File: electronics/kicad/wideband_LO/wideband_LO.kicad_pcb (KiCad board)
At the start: 2 copper layers, 27 parts, among them U1 BFP620

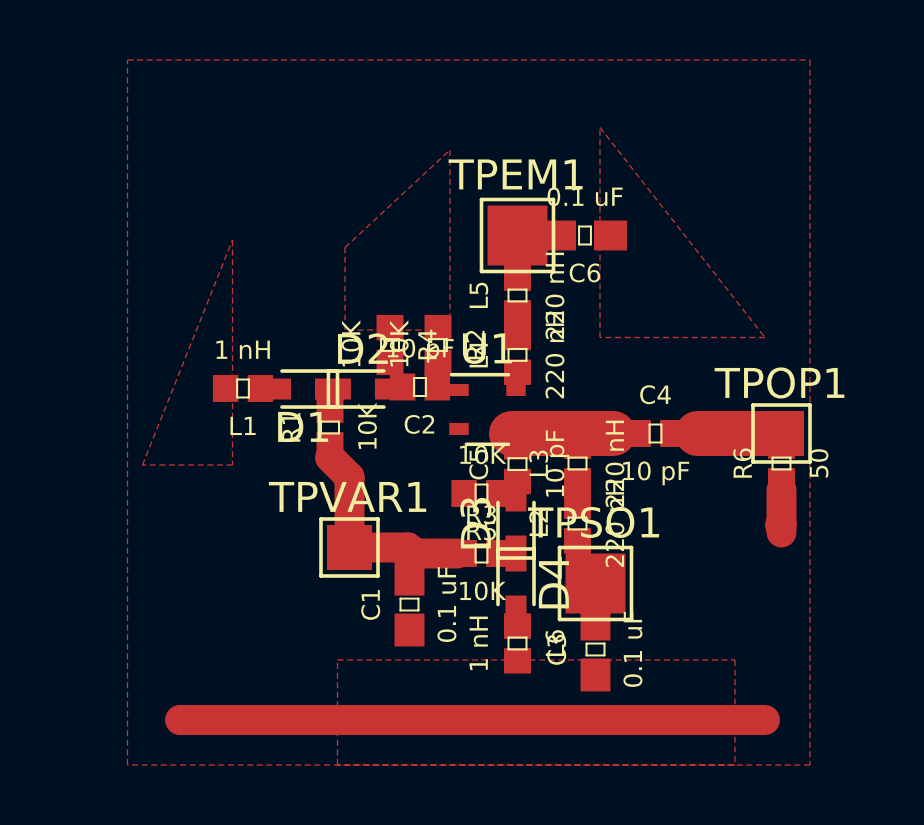
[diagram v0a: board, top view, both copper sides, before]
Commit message: Various sims
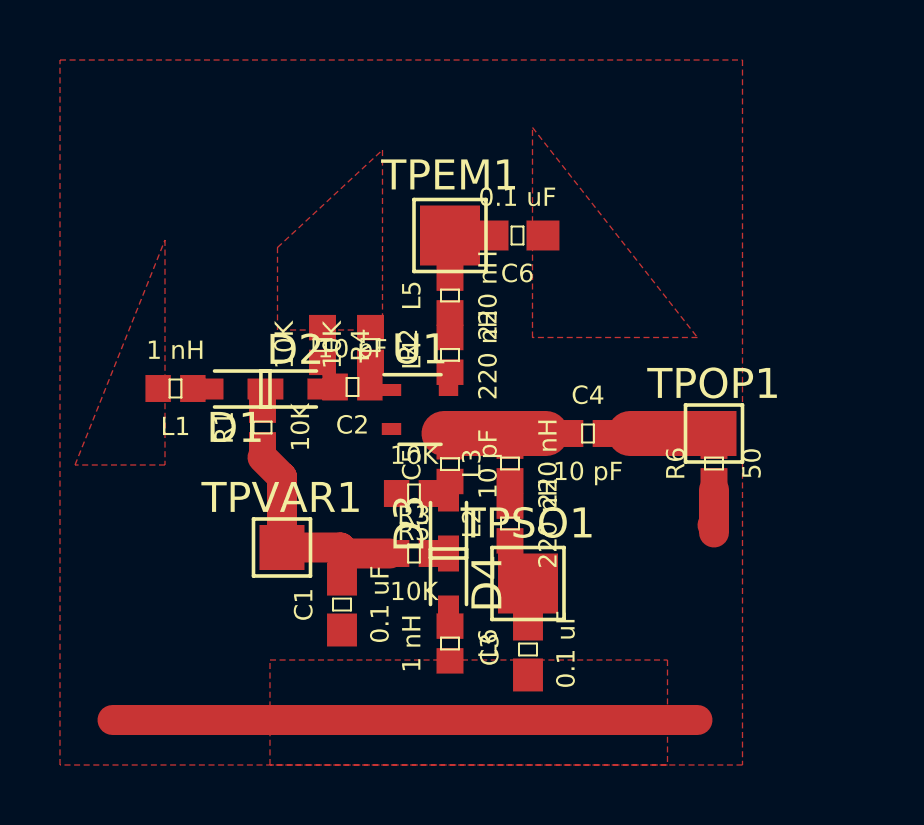
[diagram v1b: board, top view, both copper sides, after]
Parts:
- moved C1 2.25 mm to (93.2, 103.9)
- moved C2 2.25 mm to (93.5, 96.7)
- moved C3 2.25 mm to (99.3, 105.4)
- moved C4 2.25 mm to (101.3, 98.2)
- moved C5 2.25 mm to (96.8, 99.2)
- moved C6 2.25 mm to (99.0, 91.6)
- moved D1 2.25 mm to (89.6, 96.7)
- moved D2 2.25 mm to (91.6, 96.7)
- moved D3 2.25 mm to (96.7, 101.2)
- moved D4 2.25 mm to (96.7, 103.2)
- moved L1 2.25 mm to (87.6, 96.7)
- moved L2 2.25 mm to (98.8, 101.2)
- moved L3 2.25 mm to (98.8, 99.2)
- moved L4 2.25 mm to (96.8, 95.6)
- moved L5 2.25 mm to (96.8, 93.6)
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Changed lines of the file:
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@@
     (visible_elements FFFFFF7F)
     (pcbplotparams
-      (layerselection 0x010fc_ffffffff)
+      (layerselection 0x00000_7fffffff)
       (usegerberextensions false)
       (usegerberattributes false)
@@
       (creategerberjobfile false)
       (excludeedgelayer true)
-      (linewidth 0.010000)
+      (linewidth 0.020000)
       (plotframeref false)
       (viasonmask false)
       (mode 1)
-      (useauxorigin false)
+      (useauxorigin true)
       (hpglpennumber 1)
       (hpglpenspeed 20)
@@
       (outputformat 1)
       (mirror false)
-      (drillshape 1)
+      (drillshape 0)
       (scaleselection 1)
-      (outputdirectory ""))
+      (outputdirectory "CAM/"))
   )
   (net 0 "")
@@
   )
   (module Capacitors:0402 (layer F.Cu)
-    (at 107.8 99.2 90)
+    (at 105.55 99.2 90)
     (descr "GENERIC 1005 (0402) PACKAGE")
     (tags "GENERIC 1005 (0402) PACKAGE")
@@
   )
   (module Capacitors:0402 (layer F.Cu)
-    (at 97.8 100.2 180)
+    (at 95.55 100.2 180)
     (descr "GENERIC 1005 (0402) PACKAGE")
     (tags "GENERIC 1005 (0402) PACKAGE")
@@
   )
   (module Capacitors:0402 (layer F.Cu)
-    (at 94.75 95.25 270)
+    (at 92.5 95.25 270)
     (descr "GENERIC 1005 (0402) PACKAGE")
     (tags "GENERIC 1005 (0402) PACKAGE")
@@
   )
   (module Capacitors:0402 (layer F.Cu)
-    (at 97.8 102.2)
+    (at 95.55 102.2)
     (descr "GENERIC 1005 (0402) PACKAGE")
     (tags "GENERIC 1005 (0402) PACKAGE")
@@
   )
   (module Capacitors:0402 (layer F.Cu)
-    (at 96.35 95.25 270)
+    (at 94.1 95.25 270)
     (descr "GENERIC 1005 (0402) PACKAGE")
     (tags "GENERIC 1005 (0402) PACKAGE")
@@
   )
   (module Capacitors:0402 (layer F.Cu)
-    (at 92.75 98 90)
+    (at 90.5 98 90)
     (descr "GENERIC 1005 (0402) PACKAGE")
     (tags "GENERIC 1005 (0402) PACKAGE")
@@
   )
   (module Capacitors:0402 (layer F.Cu)
-    (at 99 105.2 270)
+    (at 96.75 105.2 270)
     (descr "GENERIC 1005 (0402) PACKAGE")
     (tags "GENERIC 1005 (0402) PACKAGE")
@@
   )
   (module Capacitors:0402 (layer F.Cu)
-    (at 99 93.6 90)
+    (at 96.75 93.6 90)
     (descr "GENERIC 1005 (0402) PACKAGE")
     (tags "GENERIC 1005 (0402) PACKAGE")
@@
   )
   (module Capacitors:0402 (layer F.Cu)
-    (at 99 95.57912 90)
+    (at 96.75 95.57912 90)
     (descr "GENERIC 1005 (0402) PACKAGE")
     (tags "GENERIC 1005 (0402) PACKAGE")
@@
   )
   (module Capacitors:0402 (layer F.Cu)
-    (at 101 99.2 90)
+    (at 98.75 99.2 90)
     (descr "GENERIC 1005 (0402) PACKAGE")
     (tags "GENERIC 1005 (0402) PACKAGE")
@@
   )
   (module Capacitors:0402 (layer F.Cu)
-    (at 101 101.2 90)
+    (at 98.75 101.2 90)
     (descr "GENERIC 1005 (0402) PACKAGE")
     (tags "GENERIC 1005 (0402) PACKAGE")
@@
   )
   (module Capacitors:0402 (layer F.Cu)
-    (at 89.85 96.7 180)
+    (at 87.6 96.7 180)
     (descr "GENERIC 1005 (0402) PACKAGE")
     (tags "GENERIC 1005 (0402) PACKAGE")
@@
   )
   (module Capacitors:0603 (layer F.Cu)
-    (at 101.25 91.6 180)
+    (at 99 91.6 180)
     (descr "GENERIC 1608 (0603) PACKAGE")
     (tags "GENERIC 1608 (0603) PACKAGE")
@@
   )
   (module Capacitors:0402 (layer F.Cu)
-    (at 99 99.22088 90)
+    (at 96.75 99.22088 90)
     (descr "GENERIC 1005 (0402) PACKAGE")
     (tags "GENERIC 1005 (0402) PACKAGE")
@@
   )
   (module Capacitors:0402 (layer F.Cu)
-    (at 103.6 98.2)
+    (at 101.35 98.2)
     (descr "GENERIC 1005 (0402) PACKAGE")
     (tags "GENERIC 1005 (0402) PACKAGE")
@@
   )
   (module Capacitors:0603 (layer F.Cu)
-    (at 101.6 105.4 90)
+    (at 99.35 105.4 90)
     (descr "GENERIC 1608 (0603) PACKAGE")
     (tags "GENERIC 1608 (0603) PACKAGE")
@@
   )
   (module Capacitors:0402 (layer F.Cu)
-    (at 95.75 96.65 180)
+    (at 93.5 96.65 180)
     (descr "GENERIC 1005 (0402) PACKAGE")
     (tags "GENERIC 1005 (0402) PACKAGE")
@@
   )
   (module Capacitors:0603 (layer F.Cu)
-    (at 95.4 103.90164 90)
+    (at 93.15 103.90164 90)
     (descr "GENERIC 1608 (0603) PACKAGE")
     (tags "GENERIC 1608 (0603) PACKAGE")
@@
   )
   (module TestPoint:TestPoint_Pad_1.5x1.5mm (layer F.Cu)
-    (at 93.4 102)
+    (at 91.15 102)
     (descr "SMD rectangular pad as test Point, square 1.5mm side length")
     (tags "test point SMD pad rectangle square")
@@
   )
   (module Diode_SMD:D_SOD-523 (layer F.Cu)
-    (at 93.847057 96.717156)
+    (at 91.597057 96.717156)
     (descr "http://www.diodes.com/datasheets/ap02001.pdf p.144")
     (tags "Diode SOD523")
@@
   )
   (module Diode_SMD:D_SOD-523 (layer F.Cu)
-    (at 98.95 101.2 90)
+    (at 96.7 101.2 90)
     (descr "http://www.diodes.com/datasheets/ap02001.pdf p.144")
     (tags "Diode SOD523")
@@
   )
   (module Diode_SMD:D_SOD-523 (layer F.Cu)
-    (at 91.85 96.717157 180)
+    (at 89.6 96.717157 180)
     (descr "http://www.diodes.com/datasheets/ap02001.pdf p.144")
     (tags "Diode SOD523")
@@
   )
   (module Diode_SMD:D_SOD-523 (layer F.Cu)
-    (at 98.95 103.199999 270)
+    (at 96.7 103.199999 270)
     (descr "http://www.diodes.com/datasheets/ap02001.pdf p.144")
     (tags "Diode SOD523")
@@
   )
   (module Package_TO_SOT_SMD:SOT-343_SC-70-4 (layer F.Cu)
-    (at 98 97.4)
+    (at 95.75 97.4)
     (descr "SOT-343, SC-70-4")
     (tags "SOT-343 SC-70-4")
@@
   )
   (module TestPoint:TestPoint_Pad_2.0x2.0mm (layer F.Cu)
-    (at 99 91.6)
+    (at 96.75 91.6)
     (descr "SMD rectangular pad as test Point, square 2.0mm side length")
     (tags "test point SMD pad rectangle square")
@@
   )
   (module TestPoint:TestPoint_Pad_2.0x2.0mm (layer F.Cu)
-    (at 101.6 103.2)
+    (at 99.35 103.2)
     (descr "SMD rectangular pad as test Point, square 2.0mm side length")
     (tags "test point SMD pad rectangle square")
@@
   )
   (module TestPoint:TestPoint_Pad_1.5x1.5mm (layer F.Cu)
-    (at 107.8 98.2)
+    (at 105.55 98.2)
     (descr "SMD rectangular pad as test Point, square 1.5mm side length")
     (tags "test point SMD pad rectangle square")
@@
       (net 15 noutput))
   )
-  (segment (start 87.75 107.75) (end 107.25 107.75) (width 1) (layer F.Cu) (net 1))
-  (segment (start 95.35164 102) (end 95.4 102.04836) (width 1) (layer F.Cu) (net 14))
-  (segment (start 93.4 102) (end 95.35164 102) (width 1) (layer F.Cu) (net 14))
-  (segment (start 95.55164 102.2) (end 95.4 102.04836) (width 1) (layer F.Cu) (net 14))
-  (segment (start 97 102.2) (end 95.33076 102.2) (width 1) (layer F.Cu) (net 14))
-  (segment (start 93.4 102) (end 93.4 99.65) (width 1) (layer F.Cu) (net 14))
-  (segment (start 93.4 99.65) (end 92.75 99) (width 1) (layer F.Cu) (net 14))
-  (segment (start 107.8 101.2033) (end 107.75 101.2533) (width 1) (layer F.Cu) (net 1))
-  (segment (start 107.8 100.07582) (end 107.8 101.5) (width 1) (layer F.Cu) (net 1))
-  (segment (start 107.4 98.2) (end 105 98.2) (width 1.5) (layer F.Cu) (net 15))
-  (segment (start 98.8 98.2) (end 99.49958 98.2) (width 1.5) (layer F.Cu) (net 4))
-  (segment (start 103.22088 98.2) (end 102.5467 98.2) (width 0.25) (layer F.Cu) (net 4))
-  (segment (start 102.2 98.2) (end 99.6533 98.2) (width 1.5) (layer F.Cu) (net 4))
+  (segment (start 85.5 107.75) (end 105 107.75) (width 1) (layer F.Cu) (net 1))
+  (segment (start 93.10164 102) (end 93.15 102.04836) (width 1) (layer F.Cu) (net 14))
+  (segment (start 91.15 102) (end 93.10164 102) (width 1) (layer F.Cu) (net 14))
+  (segment (start 93.30164 102.2) (end 93.15 102.04836) (width 1) (layer F.Cu) (net 14))
+  (segment (start 94.75 102.2) (end 93.08076 102.2) (width 1) (layer F.Cu) (net 14))
+  (segment (start 91.15 102) (end 91.15 99.65) (width 1) (layer F.Cu) (net 14))
+  (segment (start 91.15 99.65) (end 90.5 99) (width 1) (layer F.Cu) (net 14))
+  (segment (start 105.55 101.2033) (end 105.5 101.2533) (width 1) (layer F.Cu) (net 1))
+  (segment (start 105.55 100.07582) (end 105.55 101.5) (width 1) (layer F.Cu) (net 1))
+  (segment (start 105.15 98.2) (end 102.75 98.2) (width 1.5) (layer F.Cu) (net 15))
+  (segment (start 96.55 98.2) (end 97.24958 98.2) (width 1.5) (layer F.Cu) (net 4))
+  (segment (start 100.97088 98.2) (end 100.2967 98.2) (width 0.25) (layer F.Cu) (net 4))
+  (segment (start 99.95 98.2) (end 97.4033 98.2) (width 1.5) (layer F.Cu) (net 4))
   (zone (net 1) (net_name GND) (layer F.Cu) (hatch edge 0.508)
     (connect_pads (clearance 2))
@@
     (polygon
       (pts
-        (xy 108.75 109.25) (xy 86 109.25) (xy 86 85.75) (xy 108.75 85.75)
+        (xy 106.5 109.25) (xy 83.75 109.25) (xy 83.75 85.75) (xy 106.5 85.75)
       )
     )
@@
     (polygon
       (pts
-        (xy 106.25 109.25) (xy 93 109.25) (xy 93 105.75) (xy 106.25 105.75)
+        (xy 104 109.25) (xy 90.75 109.25) (xy 90.75 105.75) (xy 104 105.75)
       )
     )
@@
     (polygon
       (pts
-        (xy 107.25 95) (xy 101.75 95) (xy 101.75 88)
+        (xy 105 95) (xy 99.5 95) (xy 99.5 88)
       )
     )
@@
     (polygon
       (pts
-        (xy 89.5 99.25) (xy 86.5 99.25) (xy 89.5 91.75)
+        (xy 87.25 99.25) (xy 84.25 99.25) (xy 87.25 91.75)
       )
     )
@@
     (polygon
       (pts
-        (xy 96.75 94.75) (xy 93.25 94.75) (xy 93.25 92) (xy 96.75 88.75)
+        (xy 94.5 94.75) (xy 91 94.75) (xy 91 92) (xy 94.5 88.75)
       )
     )
